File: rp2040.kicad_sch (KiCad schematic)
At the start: 17 parts, among them U1 W25Q16JVSSIM, U2 RP2040

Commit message: change resistor part numbers to right sized ones
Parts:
- R15: Mouser part no. 603-MFR-25FTE52-27K -> 603-MFR-12FTF52-27K
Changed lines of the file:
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@@
 			)
 		)
-		(property "Mouser part no." " 603-MFR-25FTE52-27K"
+		(property "Mouser part no." " 603-MFR-12FTF52-27K"
 			(at 104.14 83.82 0)
 			(effects

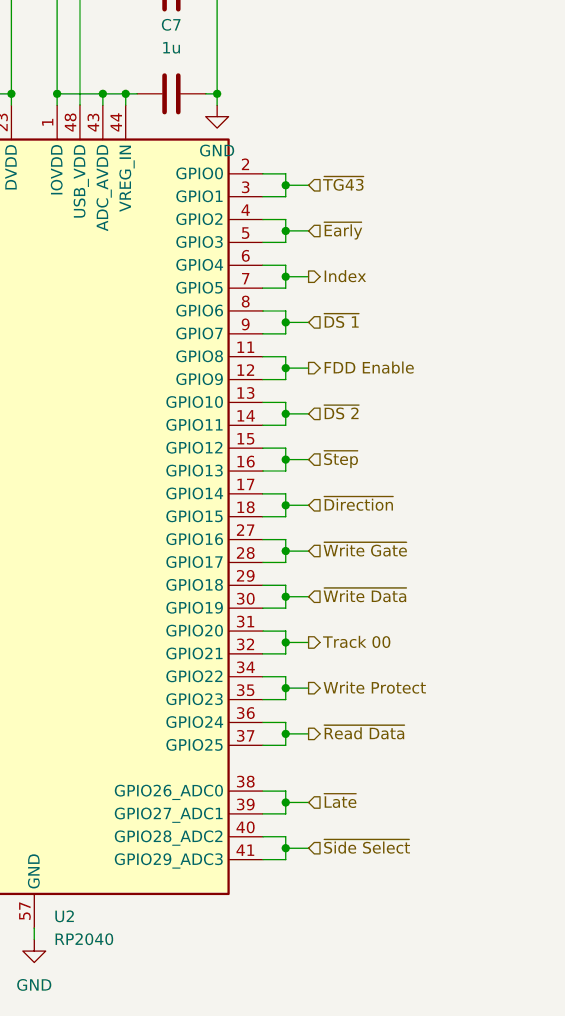
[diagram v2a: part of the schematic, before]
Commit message: Change a whole bunch of stuff for v2
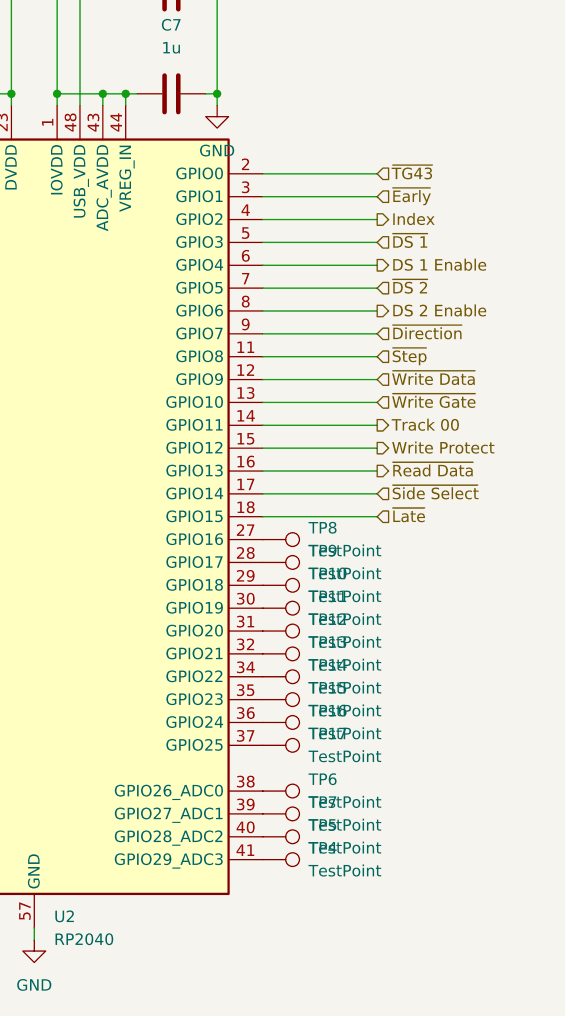
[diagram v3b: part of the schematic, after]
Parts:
- added TP10, TP11, TP12, TP13, TP14, TP15, TP16, TP17, TP4, TP5, TP6, TP7, TP8, TP9: TestPoint, symbol Connector:TestPoint
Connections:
- net Index: now also U2.4 (GPIO2); no longer U2.6 (GPIO4), U2.7 (GPIO5)
- net Track 00: now also U2.14 (GPIO11); no longer U2.31 (GPIO20), U2.32 (GPIO21)
- net Write Protect: now also U2.15 (GPIO12); no longer U2.34 (GPIO22), U2.35 (GPIO23)
- net ~{DS 1}: now also U2.5 (GPIO3); no longer U2.8 (GPIO6), U2.9 (GPIO7)
- net ~{DS 2}: now also U2.7 (GPIO5); no longer U2.13 (GPIO10), U2.14 (GPIO11)
- net ~{Direction}: now also U2.9 (GPIO7); no longer U2.17 (GPIO14), U2.18 (GPIO15)
- net ~{Early}: now also U2.3 (GPIO1); no longer U2.4 (GPIO2), U2.5 (GPIO3)
- net ~{Late}: now also U2.18 (GPIO15); no longer U2.38 (GPIO26_ADC0), U2.39 (GPIO27_ADC1)
- net ~{Read Data}: now also U2.16 (GPIO13); no longer U2.36 (GPIO24), U2.37 (GPIO25)
- net ~{Side Select}: now also U2.17 (GPIO14); no longer U2.40 (GPIO28_ADC2), U2.41 (GPIO29_ADC3)
- net ~{Step}: now also U2.11 (GPIO8); no longer U2.15 (GPIO12), U2.16 (GPIO13)
- net ~{TG43}: no longer U2.3 (GPIO1)
- net ~{Write Data}: now also U2.12 (GPIO9); no longer U2.29 (GPIO18), U2.30 (GPIO19)
- net ~{Write Gate}: now also U2.13 (GPIO10); no longer U2.27 (GPIO16), U2.28 (GPIO17)
- removed net FDD Enable: U2.11 (GPIO8), U2.12 (GPIO9)
- new net: TP7.1, U2.39 (GPIO27_ADC1)
- new net: TP4.1, U2.41 (GPIO29_ADC3)
- new net: TP6.1, U2.38 (GPIO26_ADC0)
- new net: TP15.1, U2.35 (GPIO23)
- new net: TP14.1, U2.34 (GPIO22)
- new net: TP8.1, U2.27 (GPIO16)
- new net: TP9.1, U2.28 (GPIO17)
- new net: TP10.1, U2.29 (GPIO18)
- new net: TP11.1, U2.30 (GPIO19)
- new net: TP12.1, U2.31 (GPIO20)
- new net: TP13.1, U2.32 (GPIO21)
- new net: TP16.1, U2.36 (GPIO24)
- new net: TP17.1, U2.37 (GPIO25)
- new net: TP5.1, U2.40 (GPIO28_ADC2)
- new net DS 1 Enable: U2.6 (GPIO4)
- new net DS 2 Enable: U2.8 (GPIO6)
